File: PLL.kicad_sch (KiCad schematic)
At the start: 88 parts, among them J301 Vtune, J302 RFShield_TwoPieces, J303 CPout, J304 DNP, J305 DNP, J306 DNP, J307 DNP, J308 DNP, U301 LMX2572, U302 XC6204B33

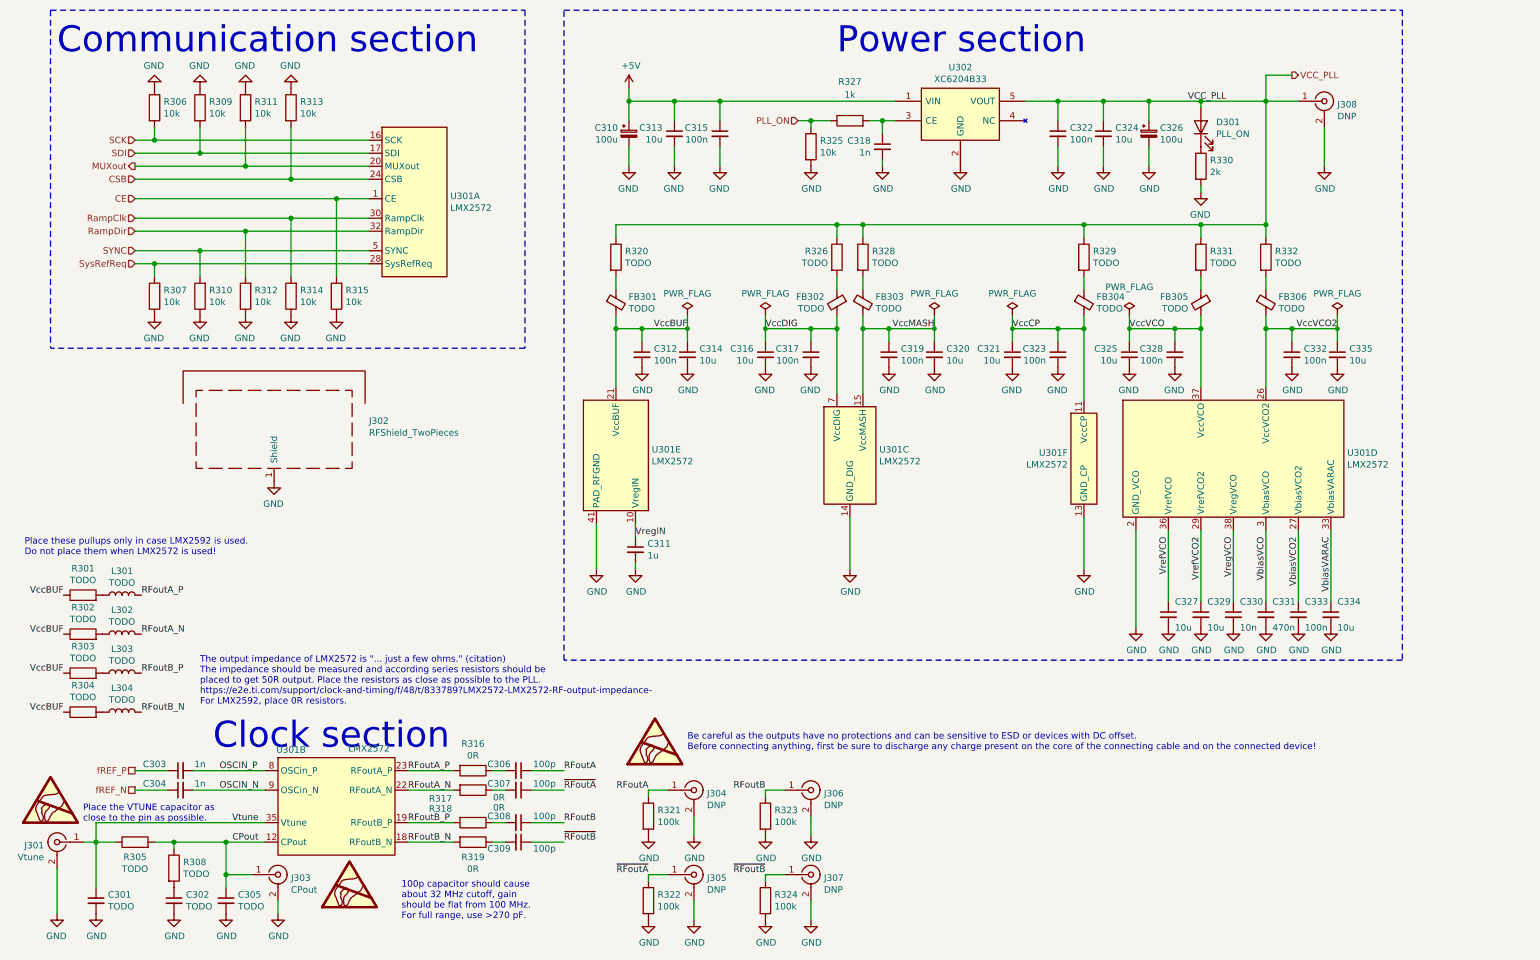
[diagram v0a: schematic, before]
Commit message: Updated schematics
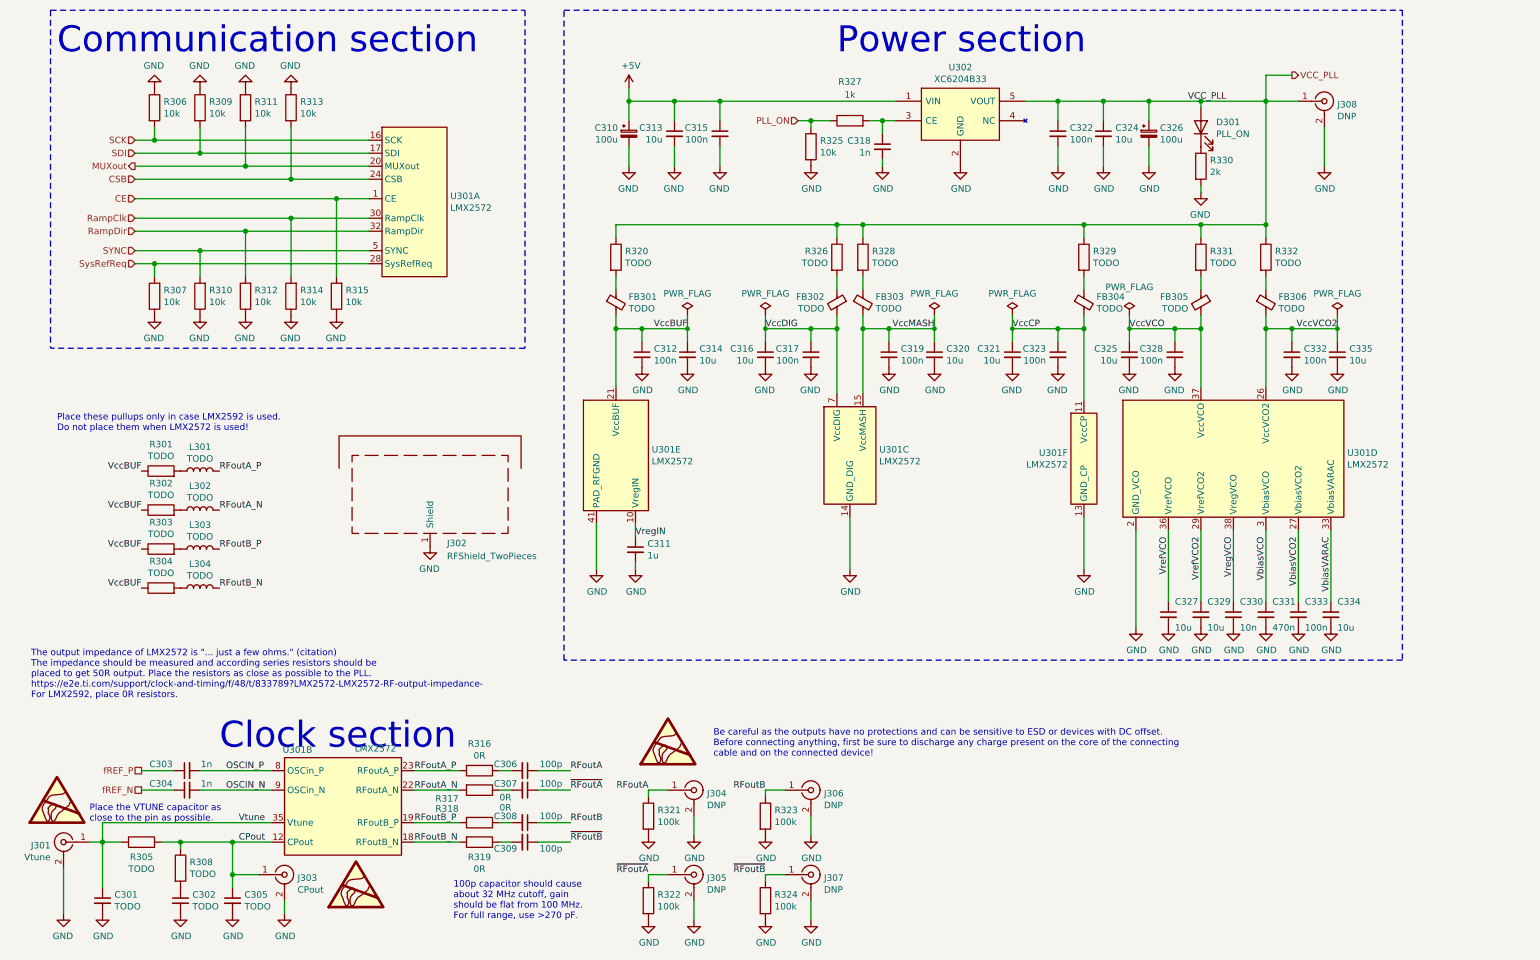
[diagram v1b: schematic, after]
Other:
- moved on the sheet: C301, C302, C303, C304, C305, C306, C307, C308, C309, J301, J302, J303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
